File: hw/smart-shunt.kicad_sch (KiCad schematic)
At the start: 43 parts, among them J1 V supply, J2 V bus <80, J3 V bus >80, J4 Conn_01x01_Female, J5 Conn_01x01_Female, J6 GND, U1 XL7005A, U2 INA228, U3 ESP-12F

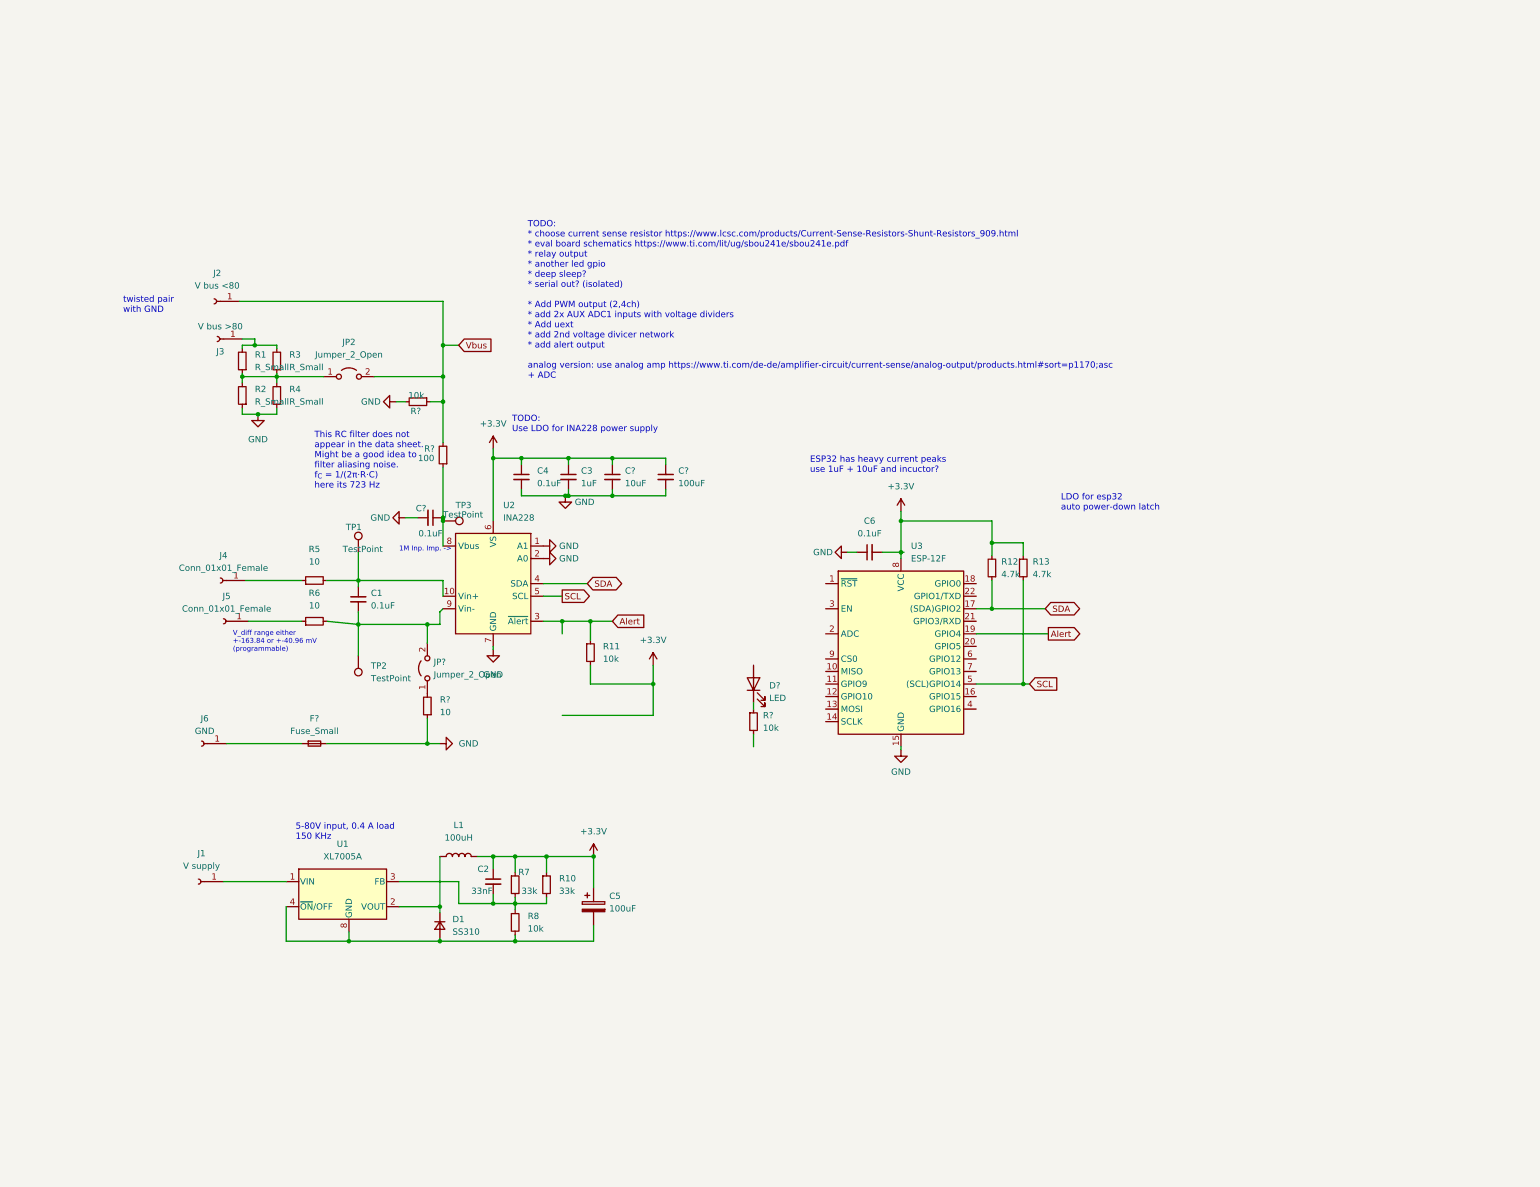
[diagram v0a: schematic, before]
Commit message: finished pcb
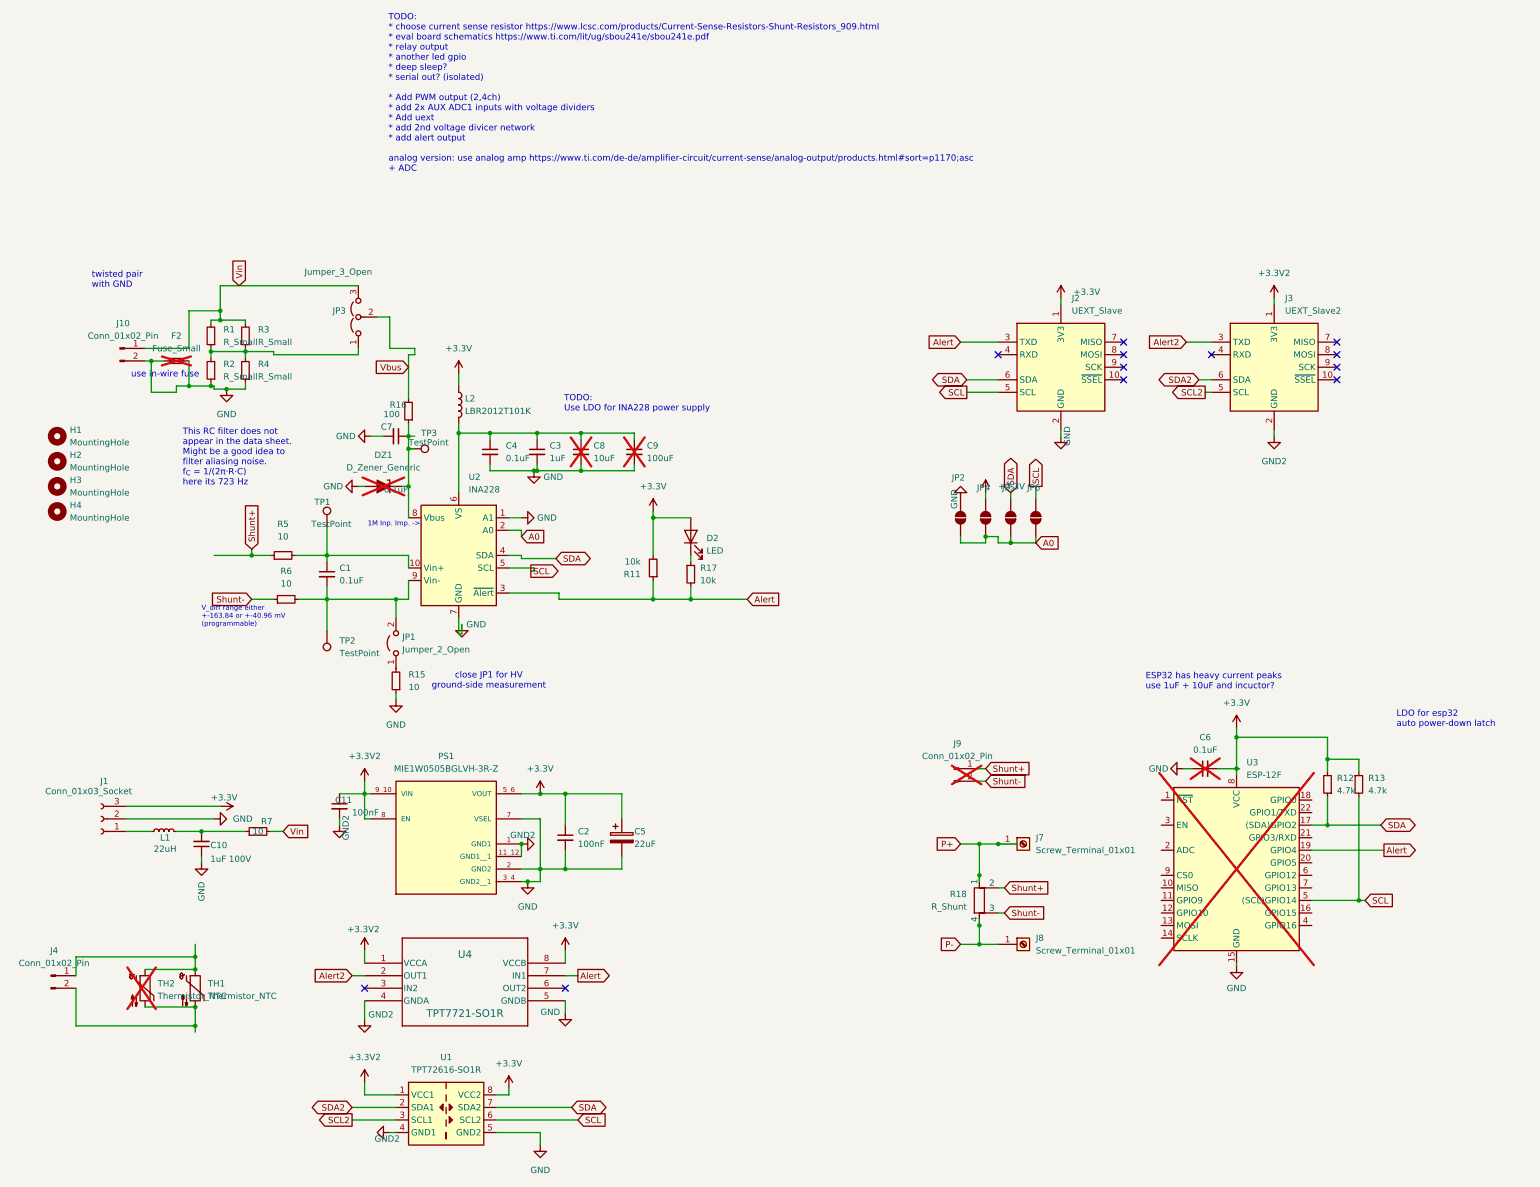
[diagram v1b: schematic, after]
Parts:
- removed D1: SS310, Diode_SMD:D_SMA_Handsoldering, symbol open-pe:SS310
- removed F?: Fuse_Small, symbol Device:Fuse_Small
- removed J1: V supply, TestPoint:TestPoint_Loop_D3.50mm_Drill0.9mm_Beaded, symbol Connector:Conn_01x01_Female
- removed J2: V bus <80, TestPoint:TestPoint_Loop_D3.50mm_Drill0.9mm_Beaded, symbol Connector:Conn_01x01_Female
- removed J3: V bus >80, TestPoint:TestPoint_Loop_D3.50mm_Drill0.9mm_Beaded, symbol Connector:Conn_01x01_Female
- removed J4, J5: Conn_01x01_Female, TestPoint:TestPoint_Loop_D3.50mm_Drill0.9mm_Beaded, symbol Connector:Conn_01x01_Female
- removed J6: GND, TestPoint:TestPoint_Loop_D3.50mm_Drill0.9mm_Beaded, symbol Connector:Conn_01x01_Female
- removed JP2: Jumper_2_Open, Jumper:SolderJumper-2_P1.3mm_Bridged2Bar_Pad1.0x1.5mm, symbol Jumper:Jumper_2_Open
- removed L1: 100uH, Inductor_SMD:L_Taiyo-Yuden_NR-60xx_HandSoldering, symbol Device:L
- removed R10: 33k, Resistor_SMD:R_0805_2012Metric, symbol Device:R_Small
- removed R8, R?: 10k, Resistor_SMD:R_0805_2012Metric, symbol Device:R_Small
- removed U1: XL7005A, Package_SO:SOIC-8_3.9x4.9mm_P1.27mm, symbol open-pe:XL7005A
- added C10: 1uF 100V, Capacitor_SMD:C_0805_2012Metric, symbol Device:C_Small
- added C11: 100nF, Capacitor_SMD:C_0805_2012Metric, symbol Device:C_Small
- added DZ1: D_Zener_Generic, symbol PCM_Diode_Zener_AKL:D_Zener_Generic
- added F2: Fuse_Small, Fuse:Fuseholder_Clip-5x20mm_Littelfuse_100_Inline_P20.50x4.60mm_D1.30mm_Horizontal, symbol Device:Fuse_Small
- added H1, H2, H3, H4: MountingHole, MountingHole:MountingHole_2.2mm_M2, symbol Mechanical:MountingHole
- added J1: Conn_01x03_Socket, Connector_PinHeader_2.54mm:PinHeader_1x03_P2.54mm_Vertical, symbol Connector:Conn_01x03_Socket
- added J10, J4, J9: Conn_01x02_Pin, Connector_PinHeader_2.54mm:PinHeader_1x02_P2.54mm_Vertical, symbol Connector:Conn_01x02_Pin
- added J2: UEXT_Slave, Connector_PinHeader_2.54mm:PinHeader_2x05_P2.54mm_Vertical, symbol Connector:UEXT_Slave
- added J3: UEXT_Slave2, Connector_PinHeader_2.54mm:PinHeader_2x05_P2.54mm_Vertical, symbol Connector:UEXT_Slave
- added J7, J8: Screw_Terminal_01x01, open-pe:Wuerth_PowerPlus_M5_Nut, symbol Connector:Screw_Terminal_01x01
- added JP2, JP4, JP5, JP6: SolderJumper_2_Open, PCM_Resistor_SMD_AKL:R_0402_1005Metric, symbol Jumper:SolderJumper_2_Open
- added JP3: Jumper_3_Open, Jumper:SolderJumper-3_P1.3mm_Open_RoundedPad1.0x1.5mm, symbol Jumper:Jumper_3_Open
- added L1: 22uH, Inductor_SMD:L_0805_2012Metric, symbol Device:L_Small
- added L2: LBR2012T101K, Inductor_SMD:L_0805_2012Metric, symbol Device:L
- added PS1: MIE1W0505BGLVH-3R-Z, open-pe:CONV_MIE1W0505BGLVH-3R-Z, symbol open-pe:MIE1W0505BGLVH-3R-Z
- added R18: R_Shunt, Resistor_SMD:R_Shunt_Isabellenhuette_BVR4026, symbol Device:R_Shunt
- added TH1, TH2: Thermistor_NTC, PCM_Resistor_SMD_AKL:R_0402_1005Metric, symbol Device:Thermistor_NTC
- added U1: TPT72616-SO1R, Package_SO:SOIC-8_3.9x4.9mm_P1.27mm, symbol Isolator:ISO1541
- added U4: TPT7721-SO1R, Package_SO:SOP-8_3.9x4.9mm_P1.27mm, symbol open-pe:TPT7721-SO1R
- C2: value 33nF -> 100nF
- C5: value 100uF -> 22uF; footprint Capacitor_SMD:CP_Elec_8x10 -> Capacitor_SMD:CP_Elec_6.3x5.9; MPN (none) -> A766EB226M1DLAE060
- C6, U3: now not fitted; now left out of the parts list
- C8, C9: renamed from C?; now not fitted; now left out of the parts list
- JP1: renamed from JP?; footprint (none) -> Jumper:SolderJumper-2_P1.3mm_Open_RoundedPad1.0x1.5mm
- R1, R2: footprint Resistor_SMD:R_0805_2012Metric -> Resistor_THT:R_Axial_DIN0204_L3.6mm_D1.6mm_P7.62mm_Horizontal
- R7: value 33k -> 10; footprint Resistor_SMD:R_0805_2012Metric -> PCM_Resistor_SMD_AKL:R_0805_2012Metric
- TP1, TP2, TP3: footprint TestPoint:TestPoint_Loop_D3.50mm_Drill0.9mm_Beaded -> TestPoint:TestPoint_Pad_D1.0mm
- gave numbers to parts that had none: 5
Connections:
- net +3.3V: now also D2.2 (A), J1.3 (Pin_3), J2.1 (3V3), JP4.2 (B), L2.1, PS1.5_6 (VOUT), U1.8 (VCC2), U4.8 (VCCB); no longer C3.1, C4.1, C8.1, C9.1, R7.1, U2.6 (VS)
- net Alert: now also R17.2, J2.3 (TXD), U4.7 (IN1)
- net GND: now also C2.2, C5.2, C10.1, DZ1.2 (A), F2.1, F2.2, J1.2 (Pin_2), J10.2 (Pin_2), J2.2 (GND), JP2.2 (B), PS1.2 (GND2), PS1.3_4 (GND2__1), PS1.7 (VSEL), U1.5 (GND2), U4.5 (GNDB); no longer U2.2 (A0)
- net SCL: now also J2.5 (SCL), JP6.2 (B), U1.6 (SCL2)
- net SDA: now also J2.6 (SDA), JP5.2 (B), U1.7 (SDA2)
- net Vbus: now also JP3.2 (C)
- net at R1.1, R2.2, R3.1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: now also JP3.1 (A)
- net Shunt-: now reaches R6.1
- net Shunt-: now also J9.2 (Pin_2), R18.3
- net at C7.1, R16.1, TP3.1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: now also DZ1.1 (K)
- net Vin: now reaches R7.2
- net Vin: now also R1.2, R3.2, J10.1 (Pin_1), JP3.3 (B); no longer C2.2
- net Shunt+: now reaches R5.1
- net Shunt+: now also J9.1 (Pin_1), R18.2
- new net: C3.1, C4.1, C8.1, C9.1, L2.2, U2.6 (VS)
- new net: J1.1 (Pin_1), L1.1
- new net: C10.2, L1.2, R7.1
- new net: J4.1 (Pin_1), TH1.1, TH2.1
- new net: J4.2 (Pin_2), TH1.2, TH2.2
- new net +3.3V2: C11.1, J3.1 (3V3), PS1.8 (EN), PS1.9_10 (VIN), U1.1 (VCC1), U4.1 (VCCA)
- new net A0: JP2.1 (A), JP4.1 (A), JP5.1 (A), JP6.1 (A), U2.2 (A0)
- new net Alert2: J3.3 (TXD), U4.2 (OUT1)
- new net GND2: C11.2, J3.2 (GND), PS1.1 (GND1), PS1.11_12 (GND1__1), U1.4 (GND1), U4.4 (GNDA)
- new net P+: J7.1 (Pin_1), R18.1
- new net P-: J8.1 (Pin_1), R18.4
- new net SCL2: J3.5 (SCL), U1.3 (SCL1)
- new net SDA2: J3.6 (SDA), U1.2 (SDA1)
- no-connect marks 0 -> 12
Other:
- note added: "close JP1 for HV ground-side measurement"
- note added: "use in-wire fuse"
- note removed: "5-80V input, 0.4 A load 150 KHz"
- moved on the sheet: C1, C3, C4, C7, D2, JP1, R1, R11, R12, R13, R15, R16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
